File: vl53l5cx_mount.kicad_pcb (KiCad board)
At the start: 2 copper layers, 12.7 x 7.9 mm, 4 parts, among them J1 Conn_01x06_MountingPin, U1 VL53L5CXV0GC/1

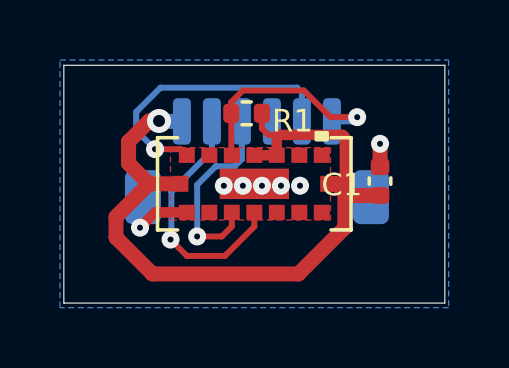
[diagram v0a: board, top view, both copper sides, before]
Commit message: update silkscreen
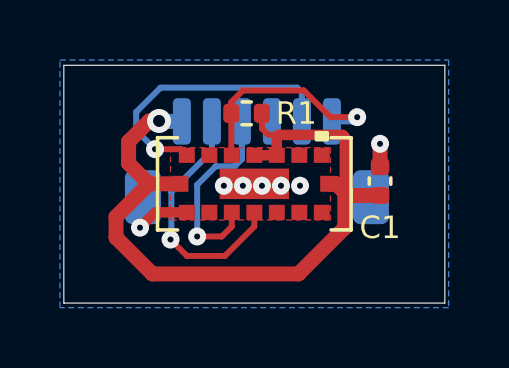
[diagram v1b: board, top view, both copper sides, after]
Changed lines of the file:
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@@
     (property "Sheetname" "")
     (attr smd)
-    (fp_text reference "C1" (at -0.127 -1.27) (layer "F.SilkS")
+    (fp_text reference "C1" (at -1.552 0) (layer "F.SilkS")
       (effects (font (size 0.75 0.75) (thickness 0.1)))
     )
@@
     (property "Sheetname" "")
     (attr smd)
-    (fp_text reference "R1" (at 1.526 0.254) (layer "F.SilkS")
+    (fp_text reference "R1" (at 1.653 0) (layer "F.SilkS")
       (effects (font (size 0.75 0.75) (thickness 0.1)))
     )
